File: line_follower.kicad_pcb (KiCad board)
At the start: 2 copper layers, 151.1 x 167.8 mm, 93 parts, among them J1 Conn_01x20_Socket, J10 Conn_01x20_Pin, J11 Conn_01x20_Pin, J12 Conn_01x02_Socket, J2 Conn_01x20_Socket, J3 Conn_01x06_Socket, J4 Conn_01x06_Socket, J5 XT60-M, J6 Conn_01x02_Socket, J7 Conn_01x02_Socket, J8 Conn_01x06_Socket, J9 Conn_01x02_Socket, SW1 SW_Push, SW3 SW_Push, SW4 SW_Push, SW5 SW_Push

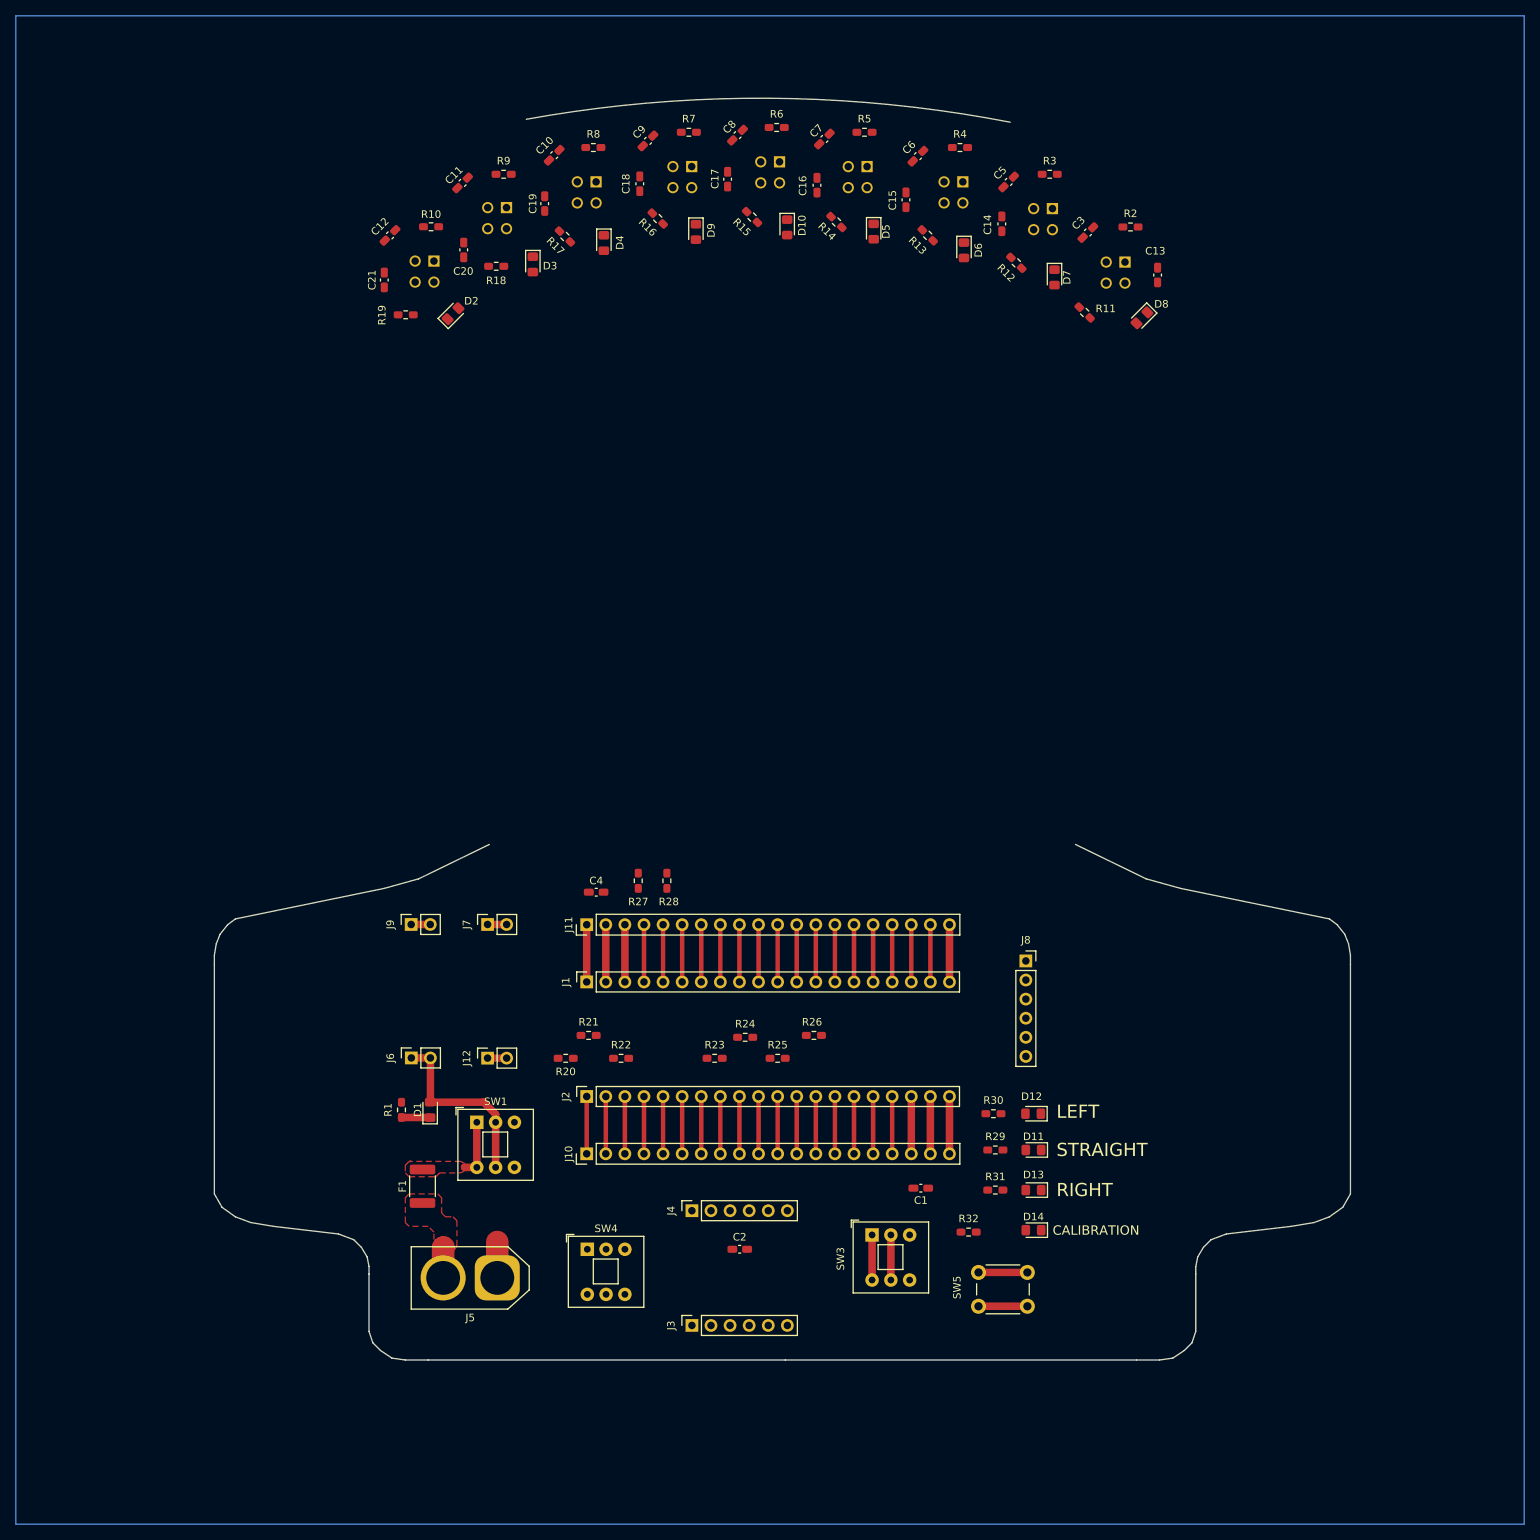
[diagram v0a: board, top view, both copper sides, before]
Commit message: minor design errors left
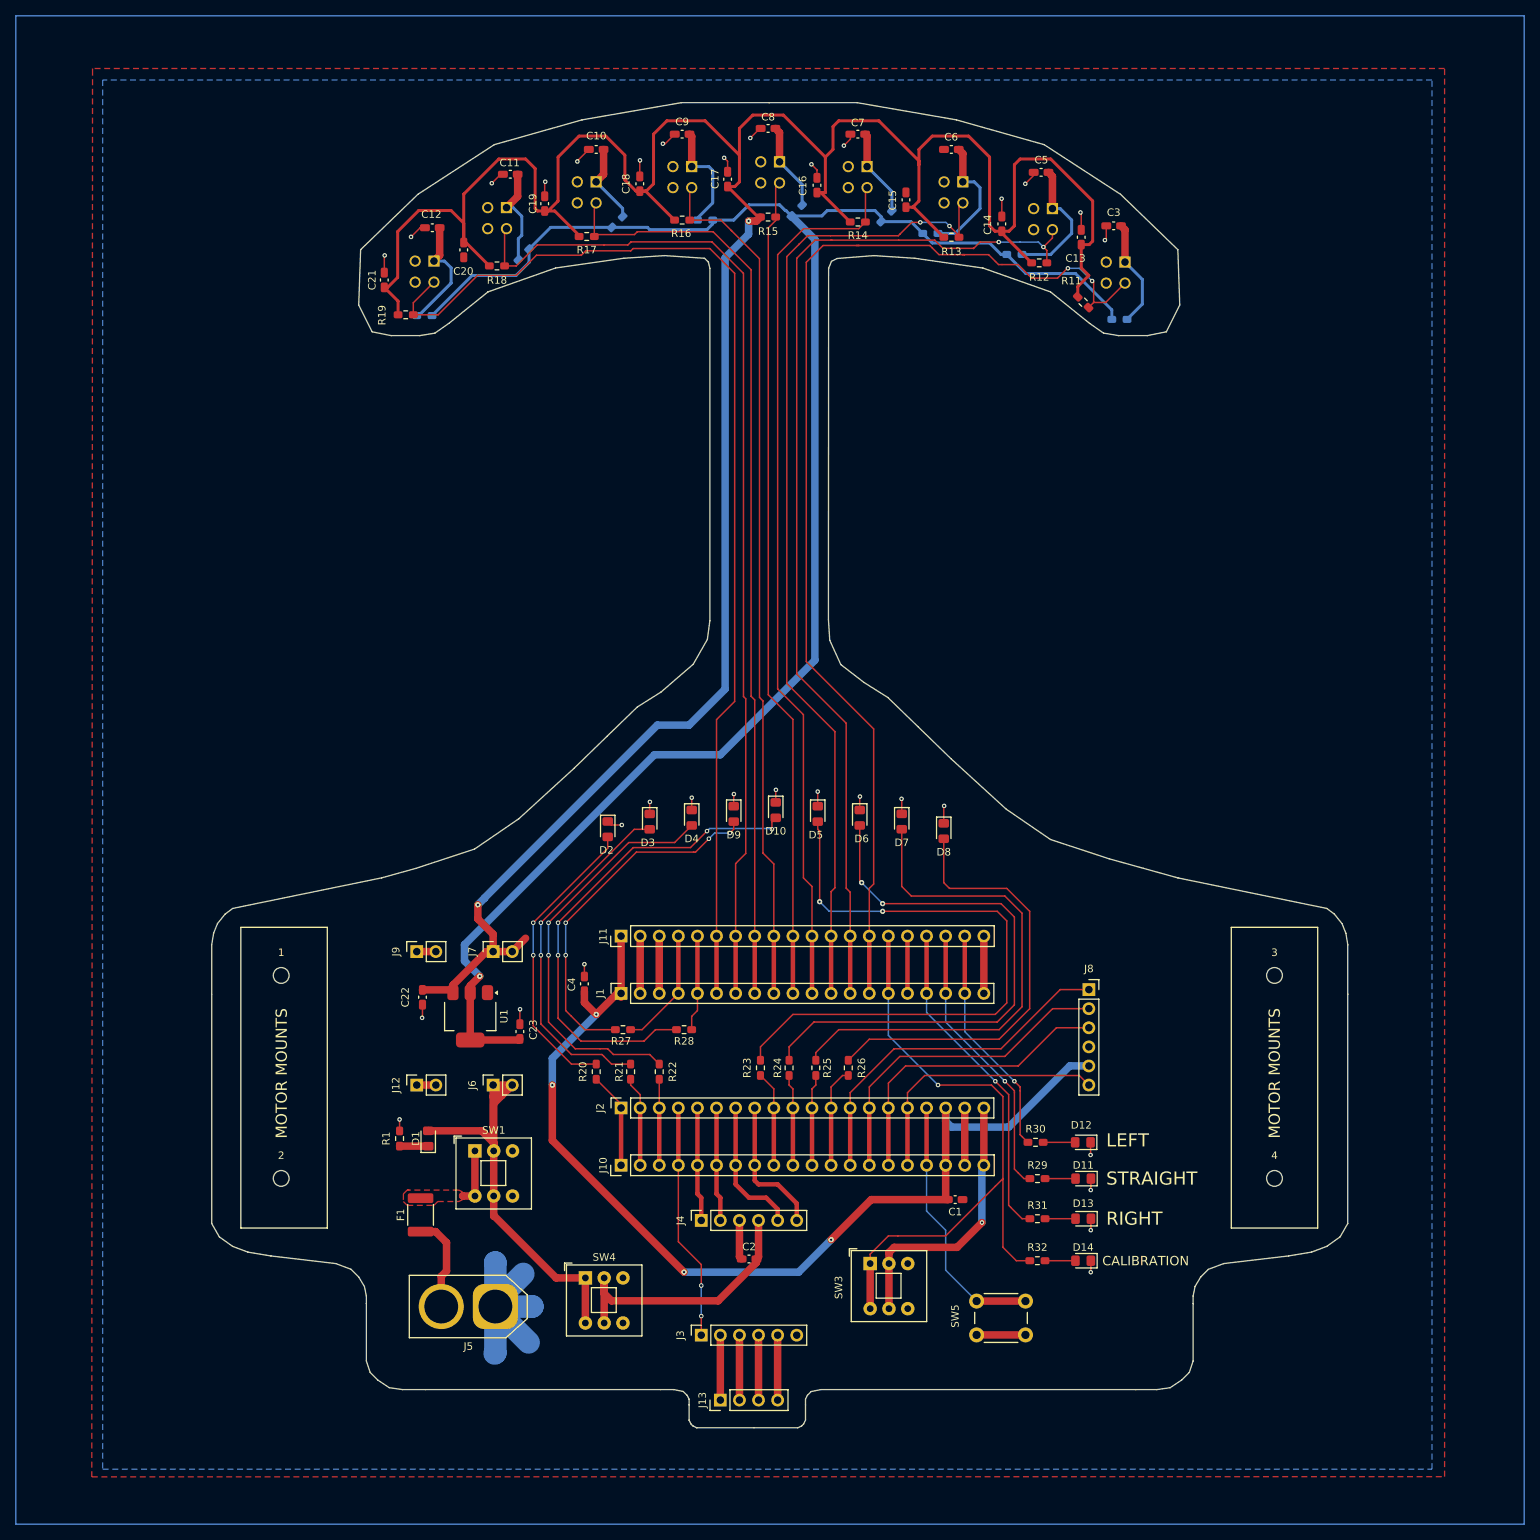
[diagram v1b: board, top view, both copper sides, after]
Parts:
- added 1: MountingHole_2.1mm, MountingHole:MountingHole_2.1mm, F.Cu at (70.9, 181.0)
- added 2: MountingHole_2.1mm, MountingHole:MountingHole_2.1mm, F.Cu at (70.9, 208.0)
- added 3: MountingHole_2.1mm, MountingHole:MountingHole_2.1mm, F.Cu at (203.0, 181.0)
- added 4: MountingHole_2.1mm, MountingHole:MountingHole_2.1mm, F.Cu at (203.0, 208.0)
- added C22: 22uf, Capacitor_SMD:C_0603_1608Metric_Pad1.08x0.95mm_HandSolder, F.Cu at (89.7, 183.9)
- added C23: 22uf, Capacitor_SMD:C_0603_1608Metric_Pad1.08x0.95mm_HandSolder, F.Cu at (102.6, 188.5)
- added J13: Conn_01x04_Pin, Connector_PinHeader_2.54mm:PinHeader_1x04_P2.54mm_Vertical, F.Cu at (129.3, 237.5)
- added U1: AMS1117-3.3, Package_TO_SOT_SMD:SOT-223-3_TabPin2, F.Cu at (96.0, 186.4)
- R10, R2, R3, R4, R5, R6, R7, R8, R9: moved to B.Cu
- moved R2 94.7 mm to (89.9, 93.2), turned to 180 degrees
- moved R10 92.4 mm to (182.4, 93.7)
- moved D5 77.8 mm to (142.2, 159.5)
- moved D9 77.6 mm to (131.1, 159.5)
- moved D10 77.5 mm to (136.7, 159.0)
- moved D4 77.3 mm to (125.5, 160.0)
- moved D6 76.8 mm to (147.8, 160.0)
- moved D3 75.7 mm to (119.9, 160.5)
- moved D7 75.2 mm to (153.4, 160.5)
- moved D8 73.2 mm to (159.0, 161.8), turned to -90 degrees
- moved D2 71.6 mm to (114.3, 161.5), turned to -90 degrees
- moved R3 70.8 mm to (103.1, 85.1), turned to -135 degrees
- moved R9 68.8 mm to (168.4, 85.1)
- moved R4 46.7 mm to (115.6, 80.8), turned to 45 degrees
- moved R8 46.3 mm to (157.2, 82.3)
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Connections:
- A1 pad 1: Net-(A1-Pad1) -> /RPR_ANO
- A2 pad 1: Net-(A2-Pad1) -> /RPR_ANO
- A3 pad 1: Net-(A3-Pad1) -> /RPR_ANO
- A4 pad 1: Net-(A4-Pad1) -> /RPR_ANO
- A5 pad 1: Net-(A5-Pad1) -> /RPR_ANO
- A6 pad 1: Net-(A6-Pad1) -> /RPR_ANO
- A7 pad 1: Net-(A7-Pad1) -> /RPR_ANO
- A8 pad 1: Net-(A8-Pad1) -> /RPR_ANO
- A9 pad 1: Net-(A9-Pad1) -> /RPR_ANO
- C10 pad 1: /3.3V_STM -> /RPR_ANO
- C11 pad 1: /3.3V_STM -> /RPR_ANO
- C12 pad 1: /3.3V_STM -> /RPR_ANO
- C3 pad 1: /3.3V_STM -> /RPR_ANO
- C5 pad 1: /3.3V_STM -> /RPR_ANO
- C6 pad 1: /3.3V_STM -> /RPR_ANO
- C7 pad 1: /3.3V_STM -> /RPR_ANO
- C8 pad 1: /3.3V_STM -> /RPR_ANO
- C9 pad 1: /3.3V_STM -> /RPR_ANO
- J1 pad 18: /LEFT -> /PC14
- J1 pad 19: /PC13 -> /LEFT
- J11 pad 18: /LEFT -> /PC14
- J11 pad 19: /PC13 -> /LEFT
- J3 pad 3: /OUT1 -> /OUT2
- J3 pad 4: /OUT1 -> /OUT3
- J3 pad 5: /OUT1 -> /OUT4
- R10 pad 2: Net-(A9-Pad1) -> /RPR_ANO
- R2 pad 2: Net-(A1-Pad1) -> /RPR_ANO
- R29 pad 1: /PB9 -> /PC14
- R3 pad 2: Net-(A2-Pad1) -> /RPR_ANO
- R31 pad 1: /PC13 -> /PC15
- R4 pad 2: Net-(A3-Pad1) -> /RPR_ANO
- R5 pad 2: Net-(A4-Pad1) -> /RPR_ANO
- R6 pad 2: Net-(A5-Pad1) -> /RPR_ANO
- R7 pad 2: Net-(A6-Pad1) -> /RPR_ANO
- R8 pad 2: Net-(A7-Pad1) -> /RPR_ANO
- R9 pad 2: Net-(A8-Pad1) -> /RPR_ANO
- SW5 pad 2: /PC15 -> /PB9
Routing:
- net /5V_STM: track 17.8 -> 528.0 mm, vias 0 -> 6
- net /3.3V_STM: track 21.2 -> 294.0 mm, vias 0 -> 2
- net /PA1: track 7.62 -> 153.0 mm, vias 0 -> 2
- net /PB1: track 7.62 -> 150.1 mm
- net /PA2: track 7.62 -> 141.0 mm, vias 0 -> 2
- net /PB0: track 7.62 -> 136.5 mm
- net /RPR_ANO: track 0.00 -> 128.0 mm
- net /PA3: track 7.62 -> 131.5 mm, vias 0 -> 2
- net /PA7: track 7.62 -> 124.2 mm
- net /PA4: track 7.62 -> 118.3 mm
- net /PA6: track 7.62 -> 114.4 mm
- net /PA5: track 7.62 -> 109.8 mm
- net GND: track 31.6 -> 123.1 mm, vias 0 -> 32
- net Net-(D5-A): track 0.00 -> 84.6 mm, vias 0 -> 2
- net Net-(D6-A): track 0.00 -> 75.7 mm, vias 0 -> 2
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- added copper zone on B.Cu, net GND
- added copper zone on F.Cu, net GND
- removed copper zone on F.Cu, net BAT+
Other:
- board size 151.1 x 167.8 mm -> 151.1 x 176.3 mm
- board text added: "MOTOR MOUNTS"
